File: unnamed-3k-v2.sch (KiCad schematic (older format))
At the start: 31 parts, among them SW1 SW_Push, U1 ATmega32U2-AU, U2 PRTR5V0U2X, Y1 Crystal_GND24_Small

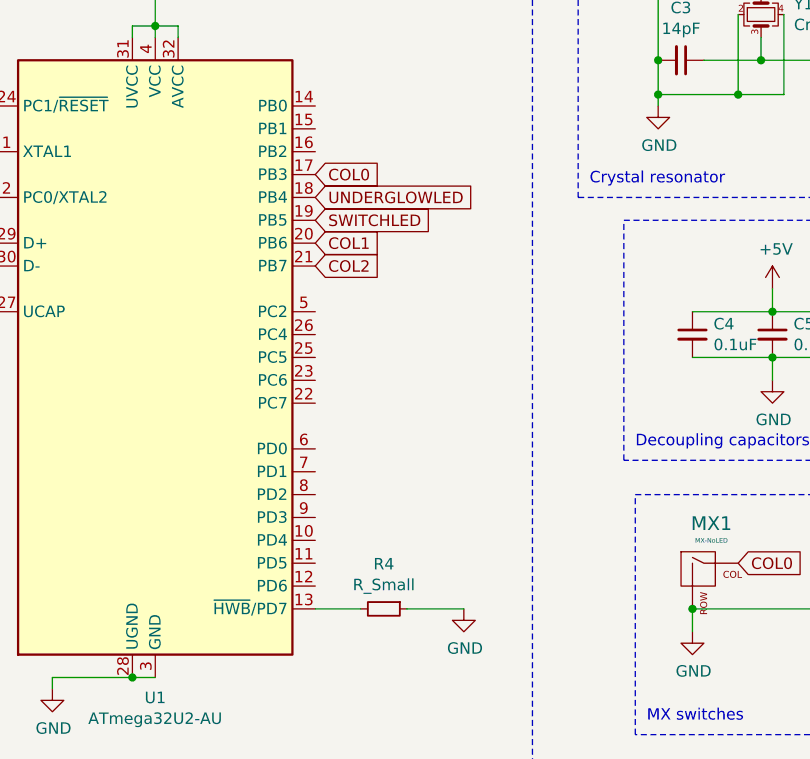
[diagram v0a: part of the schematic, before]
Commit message: everything else
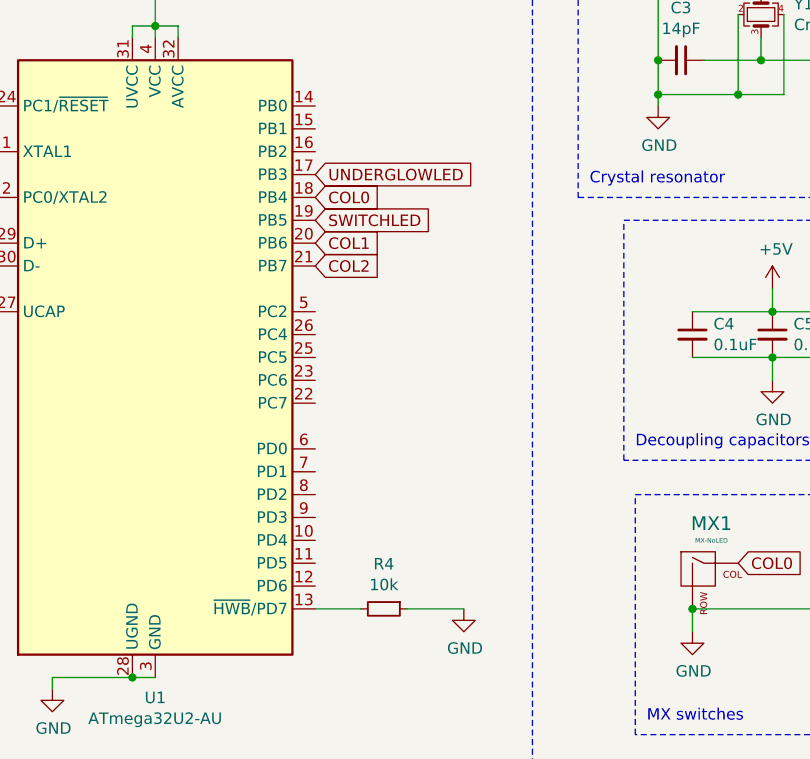
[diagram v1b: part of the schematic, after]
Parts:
- R4: value R_Small -> 10k
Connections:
- net COL0: now also U1.18 (PB4); no longer U1.17 (PB3)
- net UNDERGLOWLED: now also U1.17 (PB3); no longer U1.18 (PB4)
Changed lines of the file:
@@
 EESchema Schematic File Version 4
+LIBS:unnamed-3k-v2-cache
 EELAYER 30 0
 EELAYER END
@@
 P 4050 3700
 F 0 "R4" V 3854 3700 50  0000 C CNN
-F 1 "R_Small" V 3945 3700 50  0000 C CNN
+F 1 "10k" V 3945 3700 50  0000 C CNN
 F 2 "Resistor_SMD:R_0805_2012Metric_Pad1.15x1.40mm_HandSolder" H 4050 3700 50  0001 C CNN
 F 3 "~" H 4050 3700 50  0001 C CNN
@@
 Wire Wire Line
 	8800 3050 10050 3050
-Text GLabel 3750 1900 2    50   Input ~ 0
+Text GLabel 3750 1800 2    50   Input ~ 0
 UNDERGLOWLED
 Text GLabel 3750 2000 2    50   Input ~ 0
 SWITCHLED
-Text GLabel 3750 1800 2    50   Input ~ 0
+Text GLabel 3750 1900 2    50   Input ~ 0
 COL0
 Text GLabel 3750 2100 2    50   Input ~ 0
